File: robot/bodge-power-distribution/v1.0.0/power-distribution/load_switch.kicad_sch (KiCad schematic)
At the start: 15 parts, among them Q2 SQJA80EP-T1_GE3, Q3 SQJA80EP-T1_GE3, U1 LTC4367

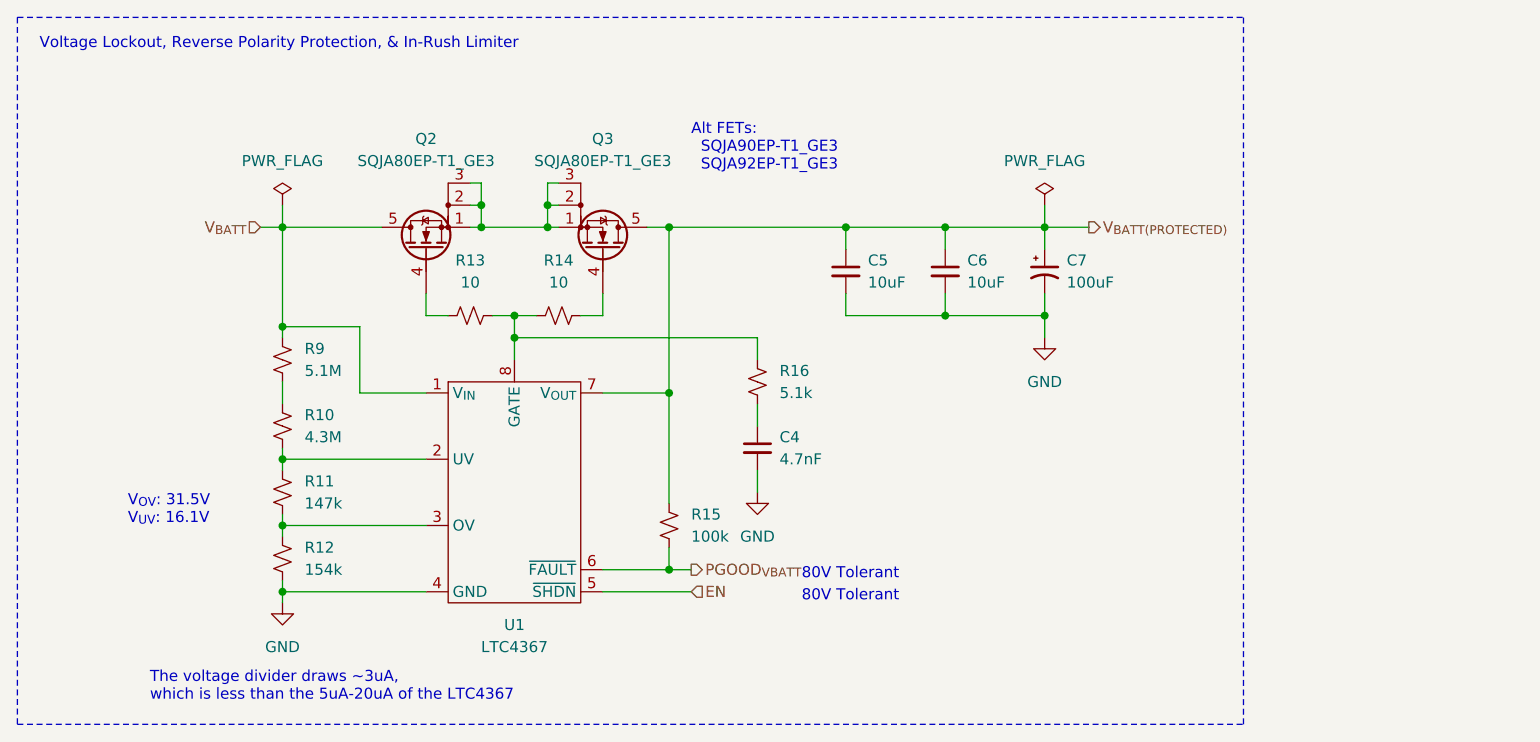
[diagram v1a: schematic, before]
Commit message: Sync
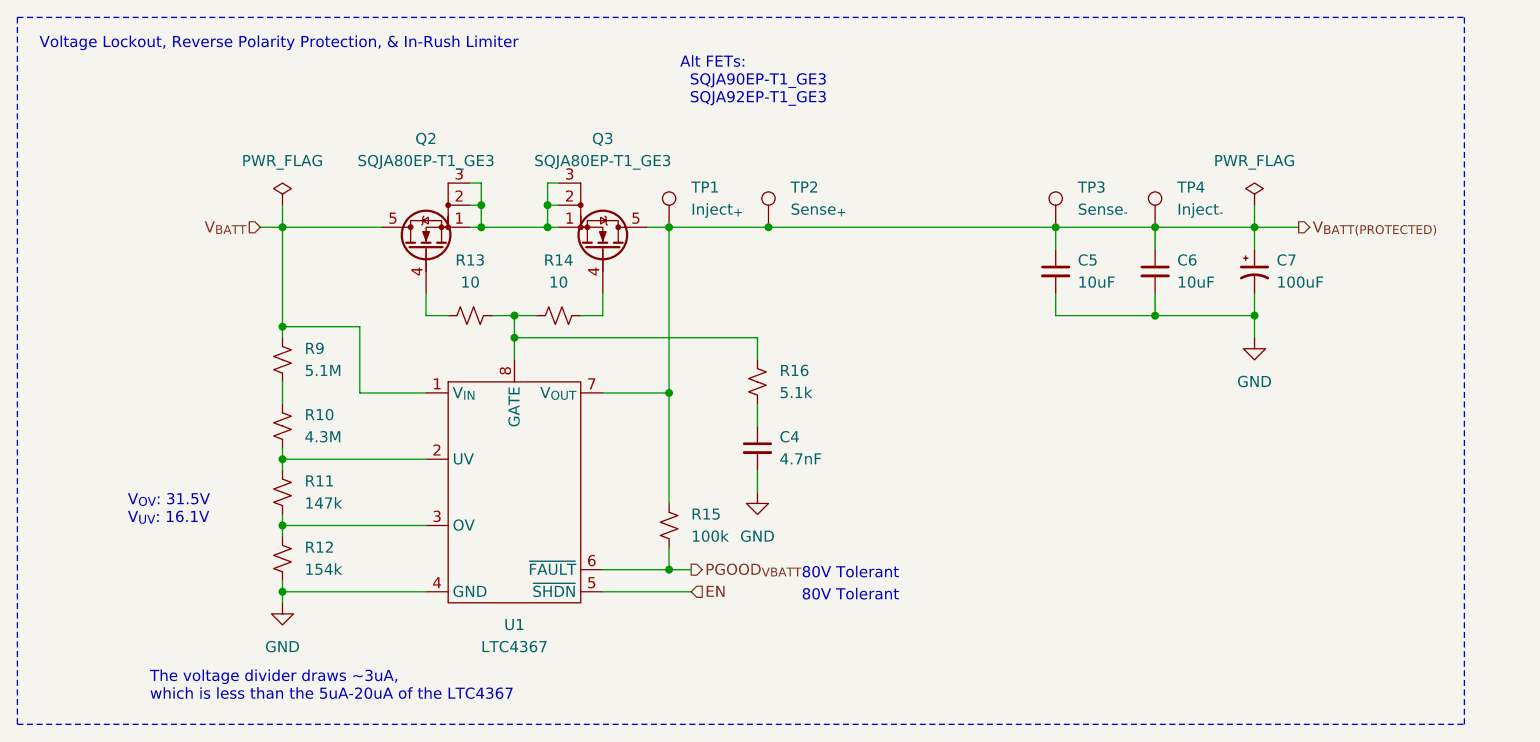
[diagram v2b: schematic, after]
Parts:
- added TP1: Inject_{+}, TestPoint:TestPoint_THTPad_2.0x2.0mm_Drill1.0mm, symbol Connector:TestPoint
- added TP2: Sense_{+}, TestPoint:TestPoint_THTPad_2.0x2.0mm_Drill1.0mm, symbol Connector:TestPoint
- added TP3: Sense_{-}, TestPoint:TestPoint_THTPad_2.0x2.0mm_Drill1.0mm, symbol Connector:TestPoint
- added TP4: Inject_{-}, TestPoint:TestPoint_THTPad_2.0x2.0mm_Drill1.0mm, symbol Connector:TestPoint
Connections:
- net V_{BATT(PROTECTED)}: now also TP1.1, TP2.1, TP3.1, TP4.1
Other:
- moved on the sheet: C5, C6, C7
